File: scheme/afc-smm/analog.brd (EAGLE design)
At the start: 100 x 80 mm, 87 parts, among them IC1 OP1177R, IC10 LM2931-5.0, IC11 OP184, IC12 DAC8551, IC13 REF3033, IC14 317EMP, IC15 317EMP, IC2 TL082D, IC3 AD8515RJ, IC4 AD8615RJ, IC5 AD8221R, IC6 AD7476, IC7 REF3033, IC8 LM337LM, IC9 317EMP, J1 22-27-2031-03, J2 22-27-2021-02, Q1 IRLML2803, X1 1-227161-0, X2 1-227161-0

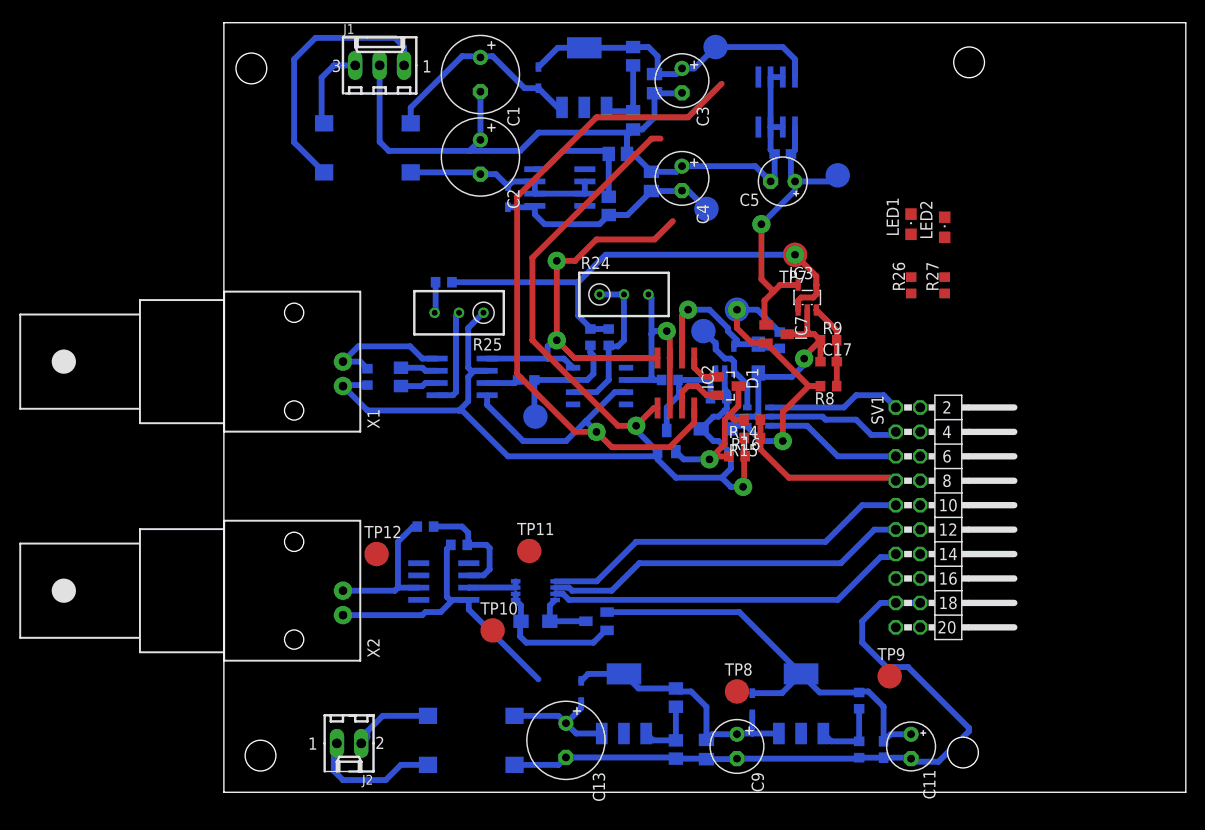
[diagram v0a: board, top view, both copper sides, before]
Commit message: compleat? version 0.1 first
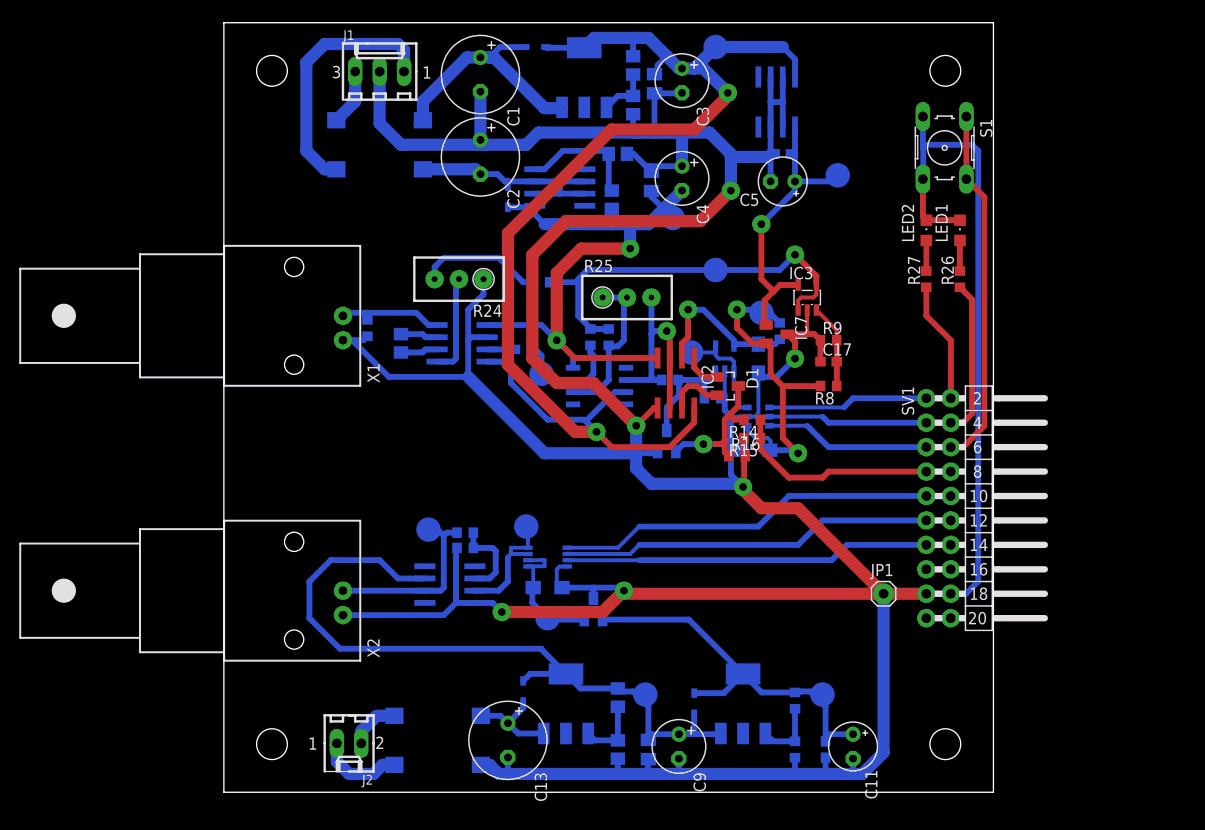
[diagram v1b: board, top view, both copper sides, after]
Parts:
- added JP1: (no value), afc-smm:1X01
- added S1: (no value), switch-omron:B3F-10XX
- R24, R25: device rcl:RTRIM3296W -> afc-smm:RTRIM3296W
- SV1: device con-lstb:MA10-2W -> afc-smm:MA10-2W
- moved R25 17.5 mm to (41.9, 51.4), turned to 270 degrees
- moved R24 17.2 mm to (24.4, 53.3), turned to 90 degrees
- moved R11 10.2 mm to (33.0, 53.0)
- moved TP8 9.53 mm to (43.8, 10.2), flipped to the bottom
- moved TP7 8.41 mm to (51.1, 54.3), flipped to the bottom
- moved TP9 7.24 mm to (62.2, 10.2), flipped to the bottom
- moved R20 6.67 mm to (59.4, 9.53)
- moved R21 6.67 mm to (59.4, 4.45)
- moved C9 6.03 mm to (47.3, 4.76)
- moved C13 6.03 mm to (29.5, 5.40)
- moved D4 6.03 mm to (31.1, 10.5)
- moved C10 6.03 mm to (44.1, 4.45)
- moved C11 6.03 mm to (65.4, 4.76)
- moved C12 6.03 mm to (62.5, 4.45)
- moved D5 6.03 mm to (48.9, 9.21)
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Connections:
- new net N$55: S1.1, S1.2, SV1.6
- net GND: now also JP1.1, R24.1, S1.3, S1.4; no longer R25.1
- net N$13: now also R25.1, R25.2; no longer R24.1, R24.2
- net N$17: now also R24.2; no longer R25.2
- net N$18: now also R24.3; no longer R25.3
- net N$9: now also R25.3; no longer R24.3
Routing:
- net GND: track 354.3 -> 507.3 mm, vias 3 -> 6
- net N$34: track 28.0 -> 75.3 mm
- net N$55: track 0.00 -> 37.3 mm
- net N$7: track 0.00 -> 15.3 mm
- net N$26: track 0.00 -> 12.6 mm
- net N$29: track 54.2 -> 44.2 mm
- net N$18: track 3.22 -> 13.1 mm
- net N$47: track 5.53 -> 13.3 mm
- net N$51: track 15.4 -> 8.80 mm
- net +12V: track 123.1 -> 128.6 mm, vias 1 -> 2
- net N$32: track 45.6 -> 40.7 mm
- net N$41: track 15.4 -> 19.4 mm
- net N$38: track 21.9 -> 25.4 mm
- net N$44: track 12.3 -> 8.84 mm
- net N$8: track 18.5 -> 21.8 mm
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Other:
- board size 100 x 80 mm -> 80 x 80 mm
